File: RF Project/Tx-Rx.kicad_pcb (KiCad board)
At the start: 2 copper layers, 30 x 55 mm, 36 parts, among them J1 CONN_Right, J2 CONN_Left, U1 CC2500RGPR, U11 Venus634SMD, U2 U.FL_male, U3 U.FL_male

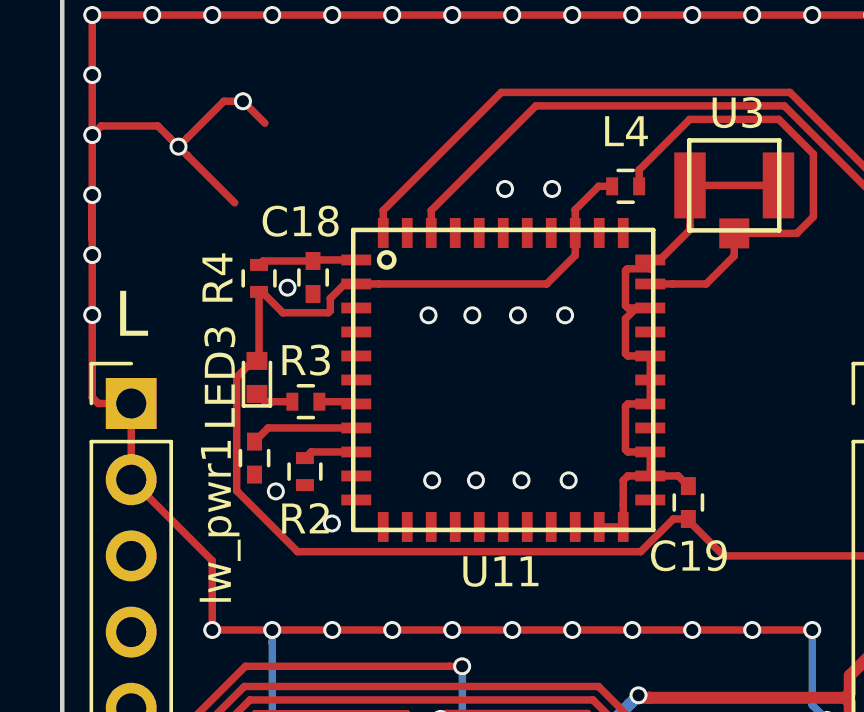
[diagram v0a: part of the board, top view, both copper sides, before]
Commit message: edit vias
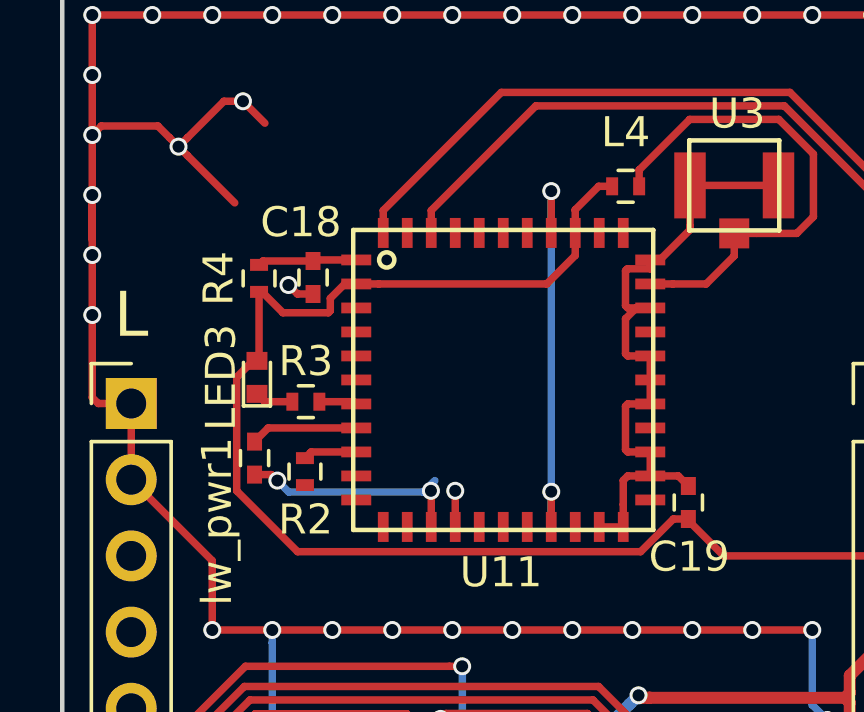
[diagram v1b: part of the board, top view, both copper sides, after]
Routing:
- net PWR_GND: track 316.8 -> 340.2 mm, vias 141 -> 134
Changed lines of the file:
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@@
   (general
     (links 106)
-    (no_connects 36)
-    (area 84.924999 72.424999 115.075001 127.575001)
+    (no_connects 12)
+    (area 60.150001 62.3 133.85 132.700001)
     (thickness 1.6)
     (drawings 27)
-    (tracks 650)
+    (tracks 657)
     (zones 0)
     (modules 36)
@@
   (segment (start 103 107.28) (end 103 107.425002) (width 0.25) (layer F.Cu) (net 7) (status 30))
   (segment (start 102.5 107.28) (end 103 107.28) (width 0.25) (layer F.Cu) (net 7) (status 30))
-  (via (at 93.99 90.45) (size 0.6) (drill 0.4) (layers F.Cu B.Cu) (net 8))
-  (via (at 92.12 89.38) (size 0.6) (drill 0.4) (layers F.Cu B.Cu) (net 8))
-  (via (at 99.76 79.3) (size 0.6) (drill 0.4) (layers F.Cu B.Cu) (net 8))
-  (via (at 101.33 79.3) (size 0.6) (drill 0.4) (layers F.Cu B.Cu) (net 8))
-  (via (at 101.76 83.51) (size 0.6) (drill 0.4) (layers F.Cu B.Cu) (net 8))
-  (via (at 100.19 83.51) (size 0.6) (drill 0.4) (layers F.Cu B.Cu) (net 8))
-  (via (at 98.67 83.51) (size 0.6) (drill 0.4) (layers F.Cu B.Cu) (net 8))
-  (via (at 97.21 83.51) (size 0.6) (drill 0.4) (layers F.Cu B.Cu) (net 8))
-  (via (at 101.88 89.01) (size 0.6) (drill 0.4) (layers F.Cu B.Cu) (net 8))
-  (via (at 100.31 89.01) (size 0.6) (drill 0.4) (layers F.Cu B.Cu) (net 8))
-  (via (at 98.79 89.01) (size 0.6) (drill 0.4) (layers F.Cu B.Cu) (net 8))
-  (via (at 92.51 82.59) (size 0.6) (drill 0.4) (layers F.Cu B.Cu) (net 8))
-  (via (at 97.33 89.01) (size 0.6) (drill 0.4) (layers F.Cu B.Cu) (net 8))
+  (segment (start 101.3 90.565) (end 101.3 89.39) (width 0.25) (layer F.Cu) (net 8))
+  (segment (start 97.3 90.565) (end 97.3 89.37) (width 0.25) (layer F.Cu) (net 8))
+  (segment (start 97.3 89.37) (end 97.29 89.36) (width 0.25) (layer F.Cu) (net 8))
+  (segment (start 101.3 79.37) (end 101.3 89.39) (width 0.25) (layer B.Cu) (net 8))
+  (segment (start 101.3 90.38) (end 101.3 89.39) (width 0.25) (layer B.Cu) (net 8))
+  (via (at 101.3 89.39) (size 0.6) (drill 0.4) (layers F.Cu B.Cu) (net 8))
+  (segment (start 101.3 80.765) (end 101.3 79.37) (width 0.25) (layer F.Cu) (net 8))
+  (via (at 101.3 79.37) (size 0.6) (drill 0.4) (layers F.Cu B.Cu) (net 8))
+  (via (at 97.29 89.36) (size 0.6) (drill 0.4) (layers F.Cu B.Cu) (net 8))
+  (segment (start 98.1 90.565) (end 98.1 89.36) (width 0.25) (layer F.Cu) (net 8))
+  (via (at 98.1 89.36) (size 0.6) (drill 0.4) (layers F.Cu B.Cu) (net 8))
+  (segment (start 97.04 89.4) (end 97.42 89.02) (width 0.25) (layer B.Cu) (net 8))
+  (segment (start 92.55 89.4) (end 97.04 89.4) (width 0.25) (layer B.Cu) (net 8))
+  (segment (start 92.17 89.02) (end 92.55 89.4) (width 0.25) (layer B.Cu) (net 8))
+  (segment (start 91.41 88.82) (end 91.97 88.82) (width 0.25) (layer F.Cu) (net 8))
+  (segment (start 91.97 88.82) (end 92.17 89.02) (width 0.25) (layer F.Cu) (net 8))
+  (via (at 92.17 89.02) (size 0.6) (drill 0.4) (layers F.Cu B.Cu) (net 8))
+  (segment (start 93.36 82.8) (end 92.84 82.8) (width 0.25) (layer F.Cu) (net 8))
+  (segment (start 92.84 82.8) (end 92.54 82.5) (width 0.25) (layer F.Cu) (net 8))
+  (via (at 92.54 82.5) (size 0.6) (drill 0.4) (layers F.Cu B.Cu) (net 8))
   (segment (start 98 105.7) (end 98 105.285134) (width 0.4) (layer F.Cu) (net 8))
   (segment (start 98 105.285134) (end 97.639246 104.92438) (width 0.4) (layer F.Cu) (net 8))
